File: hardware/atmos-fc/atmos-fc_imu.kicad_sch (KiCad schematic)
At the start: 7 parts, among them U5 ICM-42688-P

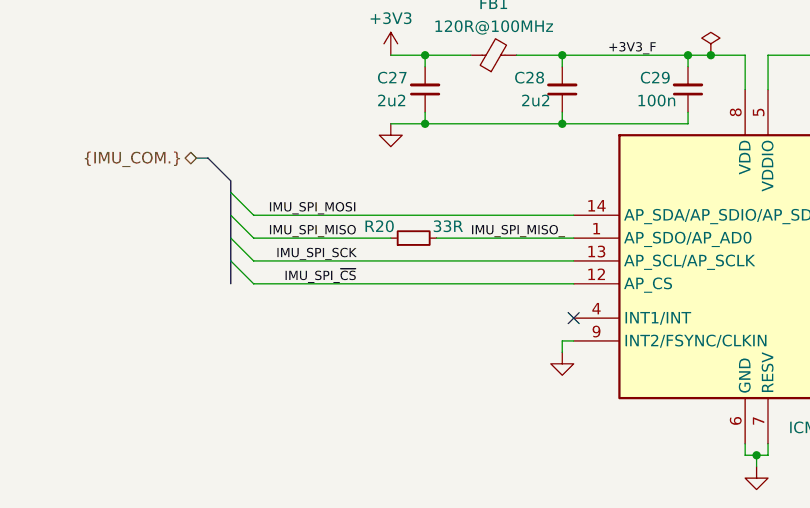
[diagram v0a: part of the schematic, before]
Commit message: Add GYRO_1_EXTI Pin
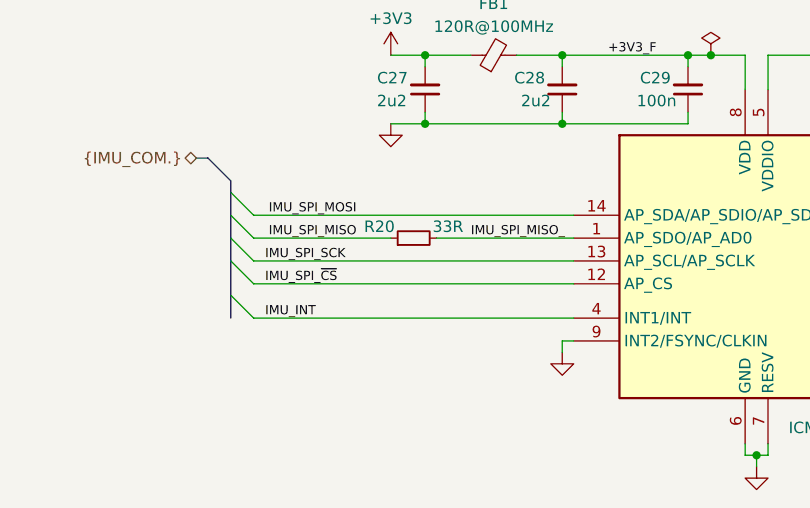
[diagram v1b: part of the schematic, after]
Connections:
- net IMU_INT: now reaches U5.4 (INT1/INT)
- no-connect marks 4 -> 3
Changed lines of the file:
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@@
-	)
-	(no_connect
-		(at 142.24 105.41)
 	)
 	(no_connect
@@
 		)
 	)
+	(bus_entry
+		(at 104.14 102.87)
+		(size 2.54 2.54)
+		(stroke
+			(width 0)
+			(type default)
+		)
+	)
 	(wire
 		(pts
@@
 	(wire
 		(pts
+			(xy 106.68 105.41) (xy 142.24 105.41)
+		)
+		(stroke
+			(width 0)
+			(type default)
+		)
+	)
+	(wire
+		(pts
 			(xy 163.83 120.65) (xy 163.83 119.38)
 		)
@@
 		)
 	)
+	(bus
+		(pts
+			(xy 104.14 102.87) (xy 104.14 105.41)
+		)
+		(stroke
+			(width 0)
+			(type default)
+		)
+	)
+	(bus
+		(pts
+			(xy 104.14 99.06) (xy 104.14 102.87)
+		)
+		(stroke
+			(width 0)
+			(type default)
+		)
+	)
 	(wire
 		(pts
@@
 		(pts
 			(xy 163.83 76.2) (xy 182.88 76.2)
-		)
-		(stroke
-			(width 0)
-			(type default)
-		)
-	)
-	(bus
-		(pts
-			(xy 104.14 99.06) (xy 104.14 101.6)
 		)
 		(stroke
@@
 		)
 	)
+	(label "IMU_INT"
+		(at 107.95 105.41 0)
+		(fields_autoplaced yes)
+		(effects
+			(font
+				(face "Arial")
+				(size 1.016 1.016)
+			)
+			(justify left bottom)
+		)
+	)
 	(label "IMU_SPI_MOSI"
 		(at 118.11 93.98 180)
@@
 	)
 	(label "IMU_SPI_SCK"
-		(at 118.11 99.06 180)
-		(fields_autoplaced yes)
-		(effects
-			(font
-				(face "Arial")
-				(size 1.016 1.016)
-			)
-			(justify right bottom)
+		(at 107.95 99.06 0)
+		(fields_autoplaced yes)
+		(effects
+			(font
+				(face "Arial")
+				(size 1.016 1.016)
+			)
+			(justify left bottom)
 		)
 	)
@@
 	)
 	(label "IMU_SPI_~{CS}"
-		(at 118.11 101.6 180)
-		(fields_autoplaced yes)
-		(effects
-			(font
-				(face "Arial")
-				(size 1.016 1.016)
-			)
-			(justify right bottom)
-		)
-	)
+		(at 107.95 101.6 0)
+		(fields_autoplaced yes)
+		(effects
+			(font
+				(face "Arial")
+				(size 1.016 1.016)
+			)
+			(justify left bottom)
+		)
+	)
